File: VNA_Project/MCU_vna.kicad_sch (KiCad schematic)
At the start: 68 parts, among them J301 2x5 1.27mm, J302 Screw_Terminal_01x02, SW301 SW_SPDT, U301 TMP75AID, U302 TMP75AID, U303 STM32H730VBTx, U304 TMP75AID, U305 TL972IPWR, Y301 STDCZS1-25M

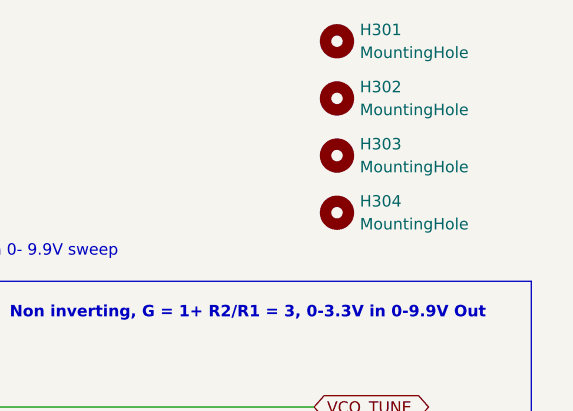
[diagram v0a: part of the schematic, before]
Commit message: Layout
Layout
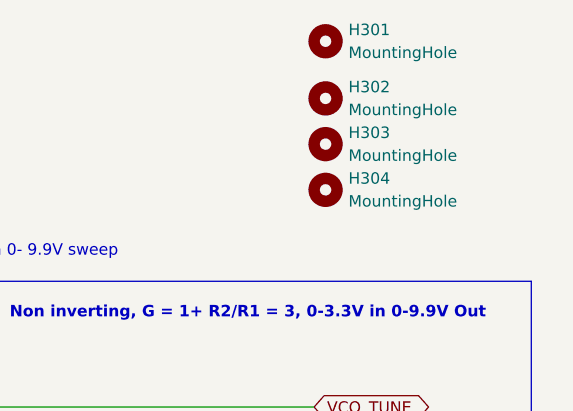
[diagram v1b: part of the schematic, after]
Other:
- moved on the sheet: H301

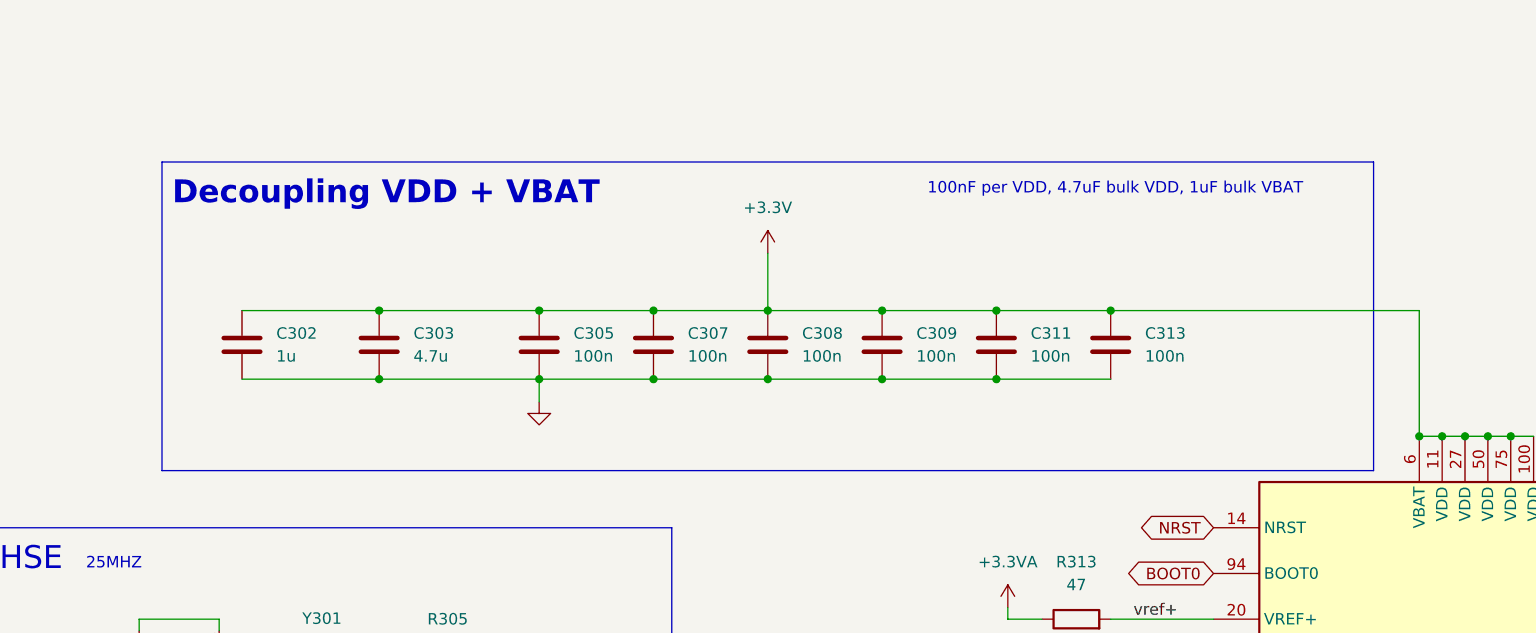
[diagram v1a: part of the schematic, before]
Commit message: minor changes
Minor Changes
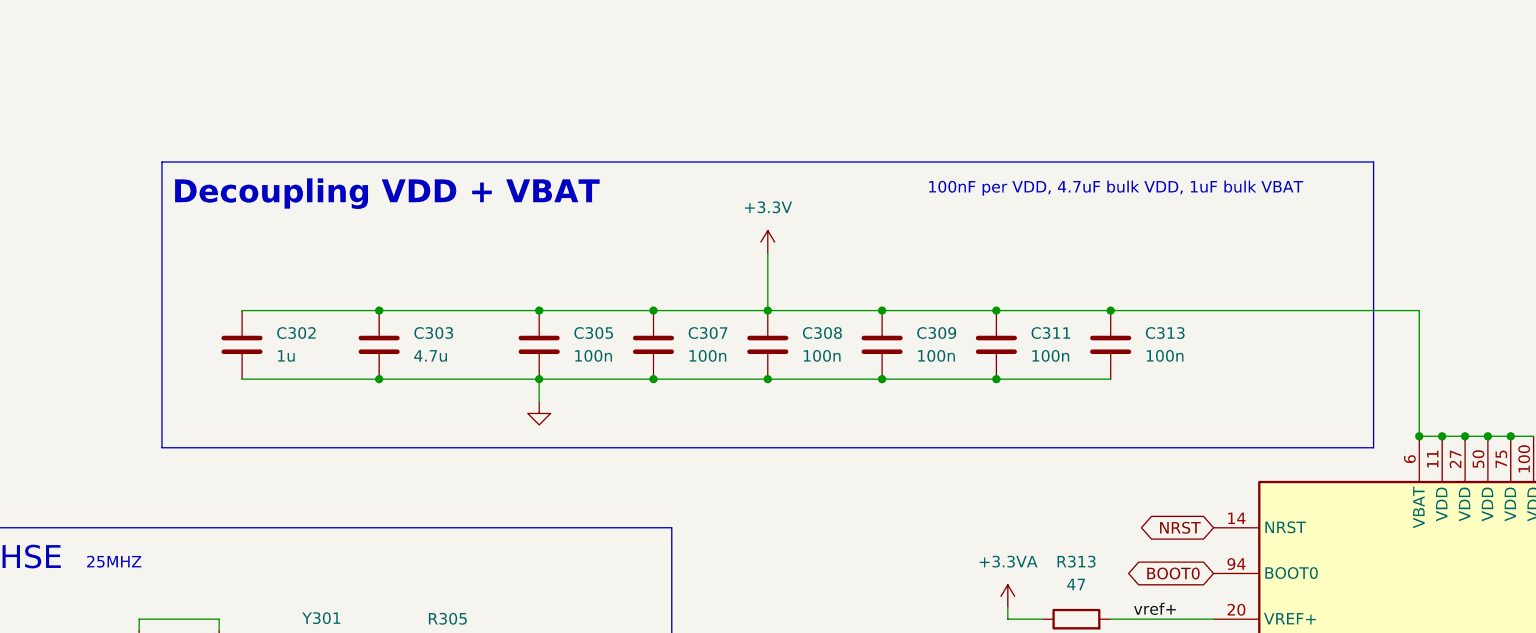
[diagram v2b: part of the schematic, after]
